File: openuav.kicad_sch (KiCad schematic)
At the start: 35 parts, among them J1 Conn_01x06, J31 Conn_01x09, J32 Conn_01x09, J33 Conn_01x09, J99 USB_C_Receptacle_USB2.0, U1 STM32G431CBUx, U3 LSM6DSR, U4 LPS22HH, U5 TPS54202DDC, U6 W25N01GVZEIG, U7 XC6206P332MR

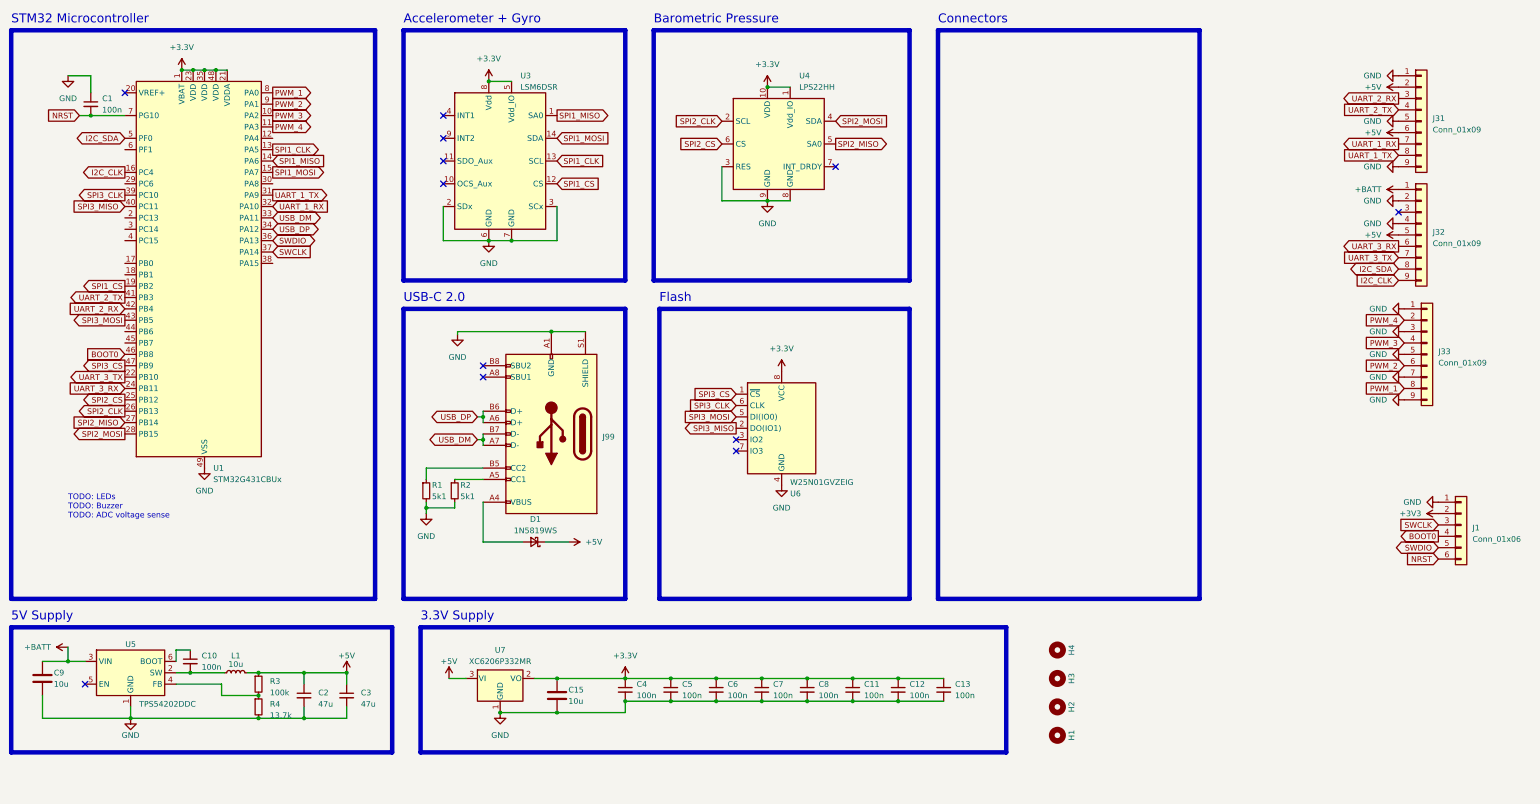
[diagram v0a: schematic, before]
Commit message: new PCB WIP
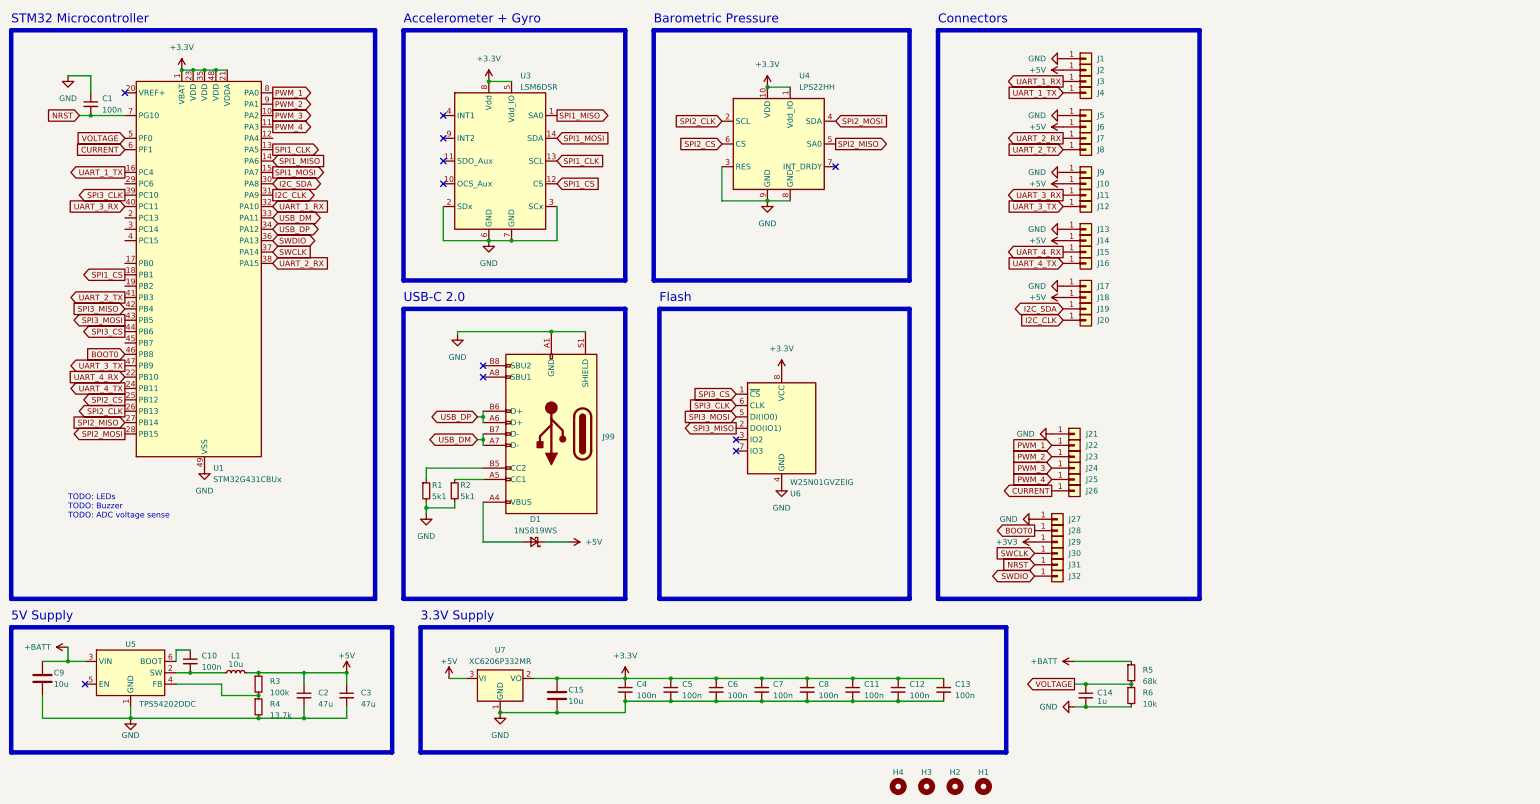
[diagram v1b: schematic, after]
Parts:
- removed J1: Conn_01x06, Connector_PinHeader_2.54mm:PinHeader_2x03_P2.54mm_Vertical, symbol Connector_Generic:Conn_01x06
- removed J31, J32, J33: Conn_01x09, Connector_PinHeader_2.54mm:PinHeader_1x09_P2.54mm_Vertical, symbol Connector_Generic:Conn_01x09
- added C14: 1u, Capacitor_SMD:C_0402_1005Metric, symbol Device:C_Small
- added J1, J10, J11, J12, J13, J14, J15, J16, J17, J18, J19, J2, J20, J21, J22, J23, J24, J25, J26, J27, J28, J29, J3, J30, J31, J32, J4, J5, J6, J7, J8, J9: Conn_01x01, TestPoint:TestPoint_THTPad_1.5x1.5mm_Drill0.7mm, symbol Connector_Generic:Conn_01x01
- added R5: 68k, Resistor_SMD:R_0402_1005Metric, symbol Device:R_Small
- added R6: 10k, Resistor_SMD:R_0402_1005Metric, symbol Device:R_Small
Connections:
- net +3V3: now also J29.1 (Pin_1)
- net +5V: now also J10.1 (Pin_1), J14.1 (Pin_1), J18.1 (Pin_1), J2.1 (Pin_1), J6.1 (Pin_1)
- net +BATT: now also R5.1
- net BOOT0: now also J28.1 (Pin_1)
- net GND: now also C14.2, J1.1 (Pin_1), J13.1 (Pin_1), J17.1 (Pin_1), J21.1 (Pin_1), J27.1 (Pin_1), J5.1 (Pin_1), J9.1 (Pin_1), R6.2
- net I2C_CLK: now also U1.31 (PA9), J20.1 (Pin_1); no longer U1.16 (PC4)
- net I2C_SDA: now also U1.30 (PA8), J19.1 (Pin_1); no longer U1.5 (PF0)
- net NRST: now also J31.1 (Pin_1)
- net PWM_1: now also J22.1 (Pin_1)
- net PWM_2: now also J23.1 (Pin_1)
- net PWM_3: now also J24.1 (Pin_1)
- net PWM_4: now also J25.1 (Pin_1)
- net SPI1_CS: now also U1.18 (PB1); no longer U1.19 (PB2)
- net SPI3_CS: now also U1.44 (PB6); no longer U1.47 (PB9)
- net SPI3_MISO: now also U1.42 (PB4); no longer U1.40 (PC11)
- net SWCLK: now also J30.1 (Pin_1)
- net SWDIO: now also J32.1 (Pin_1)
- net UART_1_RX: now also J3.1 (Pin_1)
- net UART_1_TX: now also U1.16 (PC4), J4.1 (Pin_1); no longer U1.31 (PA9)
- net UART_2_RX: now also U1.38 (PA15), J7.1 (Pin_1); no longer U1.42 (PB4)
- net UART_2_TX: now also J8.1 (Pin_1)
- net UART_3_RX: now also U1.40 (PC11), J11.1 (Pin_1); no longer U1.24 (PB11)
- net UART_3_TX: now also U1.47 (PB9), J12.1 (Pin_1); no longer U1.22 (PB10)
- net CURRENT: now reaches U1.6 (PF1)
- net CURRENT: now also J26.1 (Pin_1)
- new net UART_4_RX: J15.1 (Pin_1), U1.22 (PB10)
- new net UART_4_TX: J16.1 (Pin_1), U1.24 (PB11)
- new net VOLTAGE: C14.1, R5.2, R6.1, U1.5 (PF0)
- no-connect marks 12 -> 11
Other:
- moved on the sheet: H1, H2, H3, H4
